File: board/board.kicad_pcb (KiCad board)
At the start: 2 copper layers, 21 x 13 mm, 8 parts, among them J1 003_power, J2 003_power, U1 XC6220B331MR

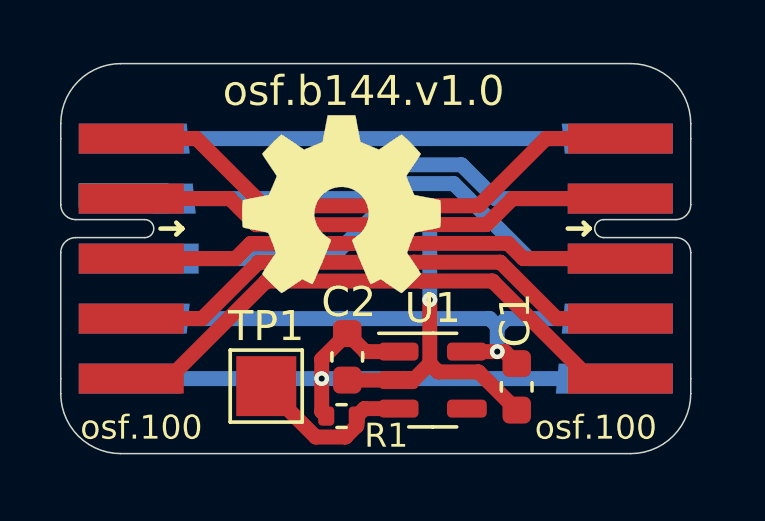
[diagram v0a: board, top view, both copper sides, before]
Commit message: V1.0
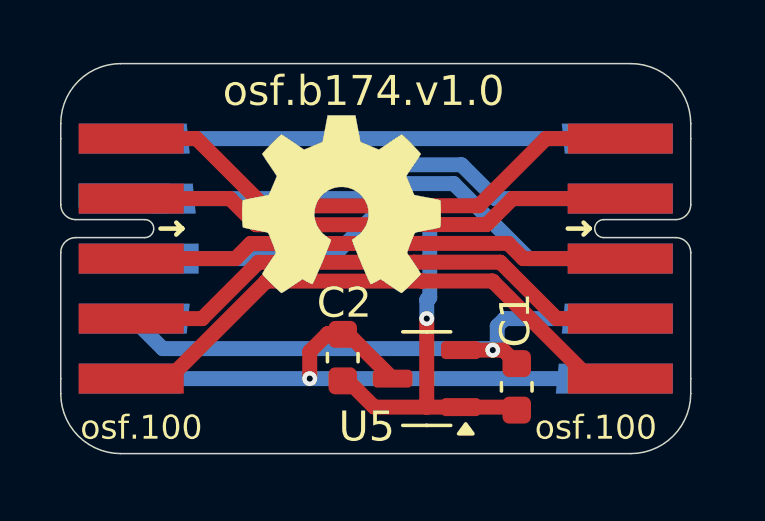
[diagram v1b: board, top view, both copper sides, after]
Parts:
- removed R1: 0R, Resistor_SMD:R_0402_1005Metric
- removed TP1: TestPoint, TestPoint:TestPoint_Pad_2.0x2.0mm
- removed U1: XC6220B331MR, Package_TO_SOT_SMD:SOT-23-5
- added U5: XC6206PxxxMR, Package_TO_SOT_SMD:SOT-23-3, F.Cu at (152.2, 100.5)
- moved C2 0.15 mm to (149.4, 99.8)
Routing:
- net /ldo/En: track 5.72 -> 0.00 mm
- net GND: track 29.9 -> 31.1 mm
- net /ldo/3.3v: track 19.1 -> 19.7 mm
- net /ldo/In: track 21.3 -> 20.8 mm
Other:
- board text added: "osf.b174.v1.0"
- board text removed: "osf.b144.v1.0"
